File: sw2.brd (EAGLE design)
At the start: 43.3 x 87 mm, 12 parts, among them X3 22-23-2041

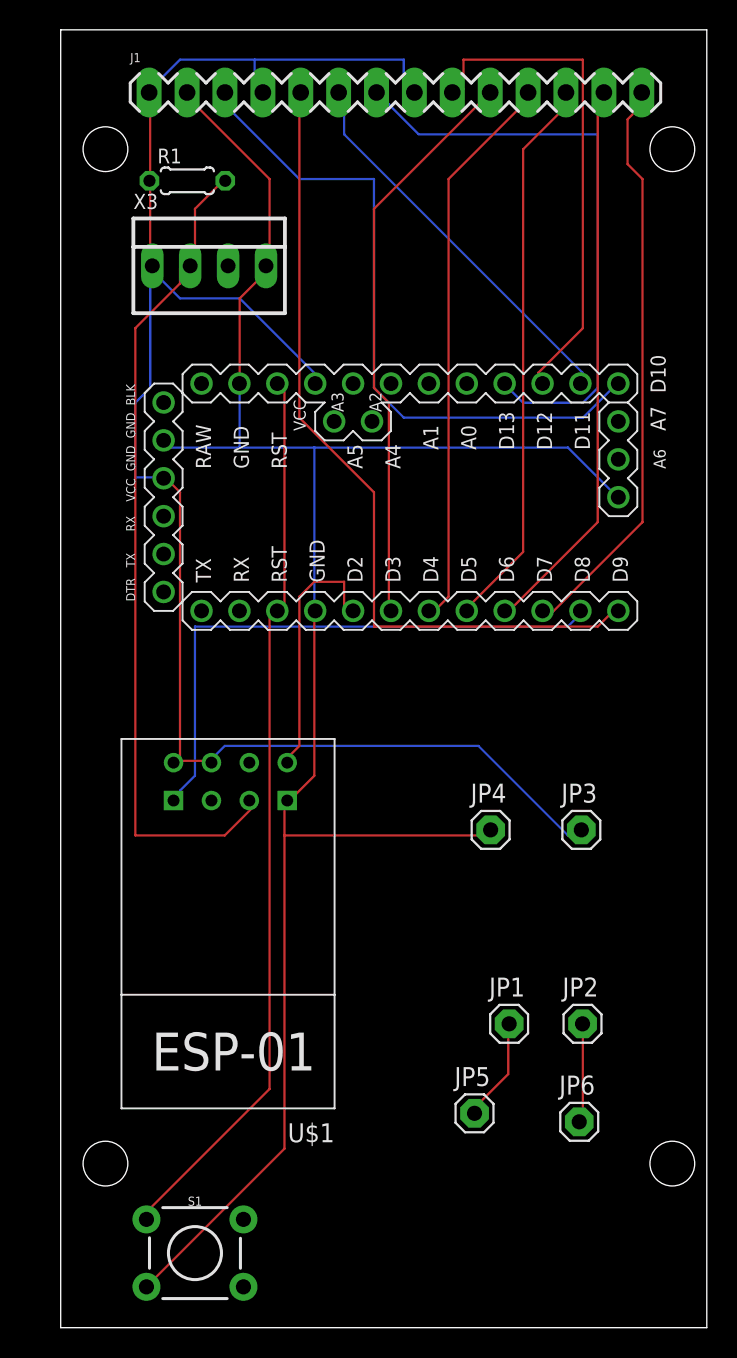
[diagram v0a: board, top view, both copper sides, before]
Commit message: Add files via upload
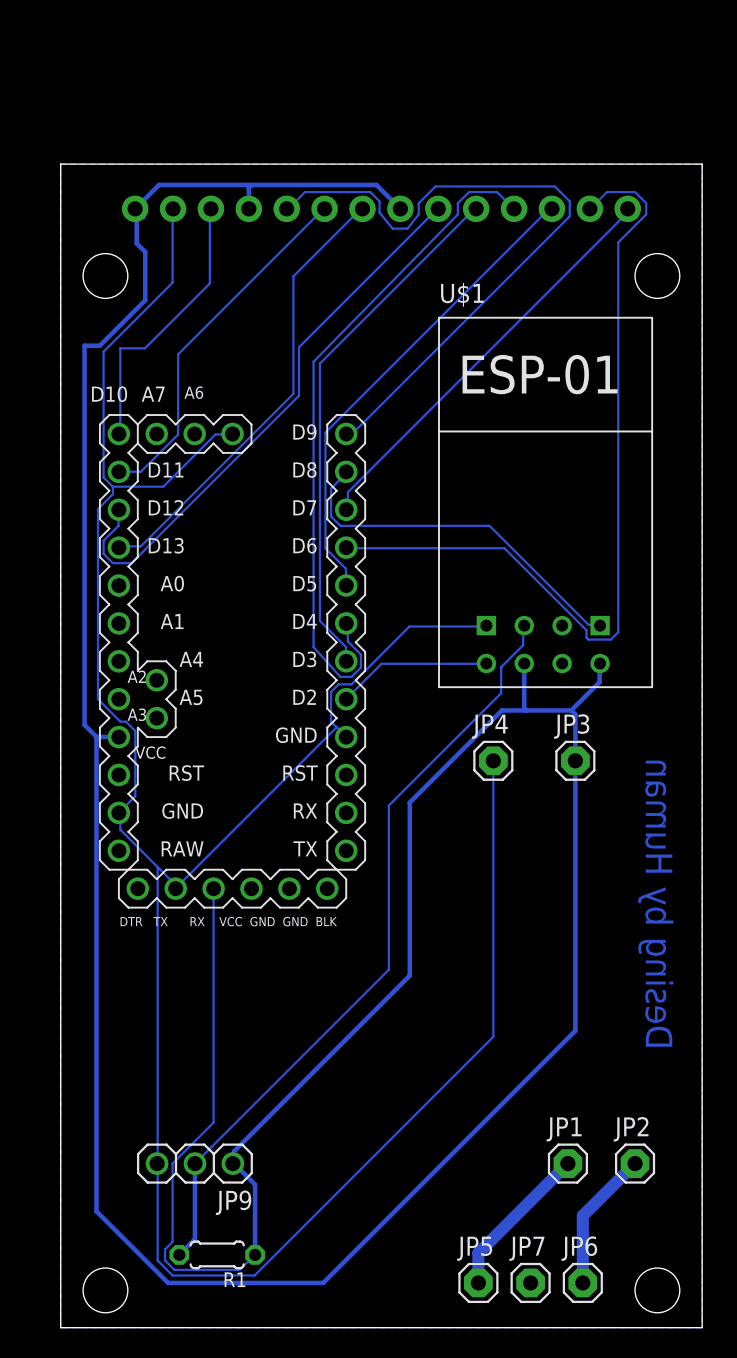
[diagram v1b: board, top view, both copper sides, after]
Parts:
- removed J1: (no value), SparkFun-Connectors:1X14-LONGPADS
- removed S1: MOMENTARY-SWITCH-SPST-PTH-6.0MM-KIT, SparkFun-Switches:TACTILE_SWITCH_PTH_6.0MM_KIT
- removed X3: 22-23-2041, con-molex:22-23-2041
- added JP7: (no value), adafruit:1X01
- added JP8: (no value), adafruit:1X14-CB
- added JP9: (no value), adafruit:1X03
- moved R1 72.0 mm to (10.5, 4.88), turned to 180 degrees
- moved U$1 31.1 mm to (32.4, 52.7), turned to 0 degrees
- moved ARDUINO1 11.4 mm to (15.3, 40.9), turned to 180 degrees
- moved JP5 11.4 mm to (28.0, 3.00)
- moved JP6 10.8 mm to (35.0, 3.00)
- moved JP1 10.2 mm to (34.0, 11.0)
- moved JP2 10.0 mm to (38.5, 11.0)
- moved JP3 4.65 mm to (34.5, 38.0)
- moved JP4 4.63 mm to (29.0, 38.0)
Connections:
- removed net N$18: ARDUINO1.RST, ARDUINO1.RST@1, S1.1
- removed net N$3 (its old number): ARDUINO1.VCC, ARDUINO1.VCC@1, J1.1, J1.4, J1.8, JP3.1, R1.1, U$1.RST, U$1.VCC, X3.1
- removed net N$4: ARDUINO1.GND, ARDUINO1.GND@1, ARDUINO1.GND@2, ARDUINO1.GND@3, J1.2, JP4.1, S1.3, U$1.GND, X3.4
- new net GND: ARDUINO1.GND, ARDUINO1.GND@1, ARDUINO1.GND@2, ARDUINO1.GND@3, JP4.1, JP8.2, JP9.3, U$1.GND
- new net VCC: ARDUINO1.VCC, ARDUINO1.VCC@1, JP3.1, JP8.1, JP8.4, JP8.8, JP9.1, R1.1, U$1.CH_PD, U$1.VCC
- net N$11: now also JP8.6; no longer J1.6
- net N$12: now also JP8.9; no longer J1.9
- net N$13: now also JP8.10; no longer J1.10
- net N$14: now also JP8.11; no longer J1.11
- net N$15: now also JP8.12; no longer J1.12
- net N$16: now also JP8.13; no longer J1.13
- net N$17: now also JP8.14; no longer J1.14
- net N$5: now also JP8.3; no longer J1.3
- net N$6: now also JP9.2; no longer X3.2
- net N$7: now also JP8.7; no longer J1.7
- net N$8: now also JP8.5; no longer J1.5
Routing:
- net VCC: track 0.00 -> 246.5 mm
- net GND: track 0.00 -> 166.5 mm
- net N$4: track 134.6 -> 0.00 mm
- net N$3 (its old number): track 116.7 -> 0.00 mm
- net N$18: track 60.7 -> 0.00 mm
- net N$5: track 45.0 -> 18.7 mm
- net N$16: track 37.6 -> 55.4 mm
- net N$10: track 39.5 -> 24.5 mm
- net N$17: track 38.8 -> 28.0 mm
- net N$7: track 40.2 -> 30.3 mm
- net N$8: track 54.7 -> 45.1 mm
- net N$14: track 37.7 -> 45.9 mm
- net N$3: track 17.7 -> 10.4 mm
- net N$15: track 37.9 -> 32.2 mm
- net N$6: track 56.1 -> 51.9 mm
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- added copper zone on layer 16, net GND
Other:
- board size 43.3 x 87 mm -> 43 x 78 mm
- board text added: "Desing by Human"
